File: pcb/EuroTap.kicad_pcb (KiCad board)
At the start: 2 copper layers, 34 x 17 mm, 5 parts, among them J1 AudioJack3_Ground, J2 AudioJack3_Ground, J3 Conn_Coaxial

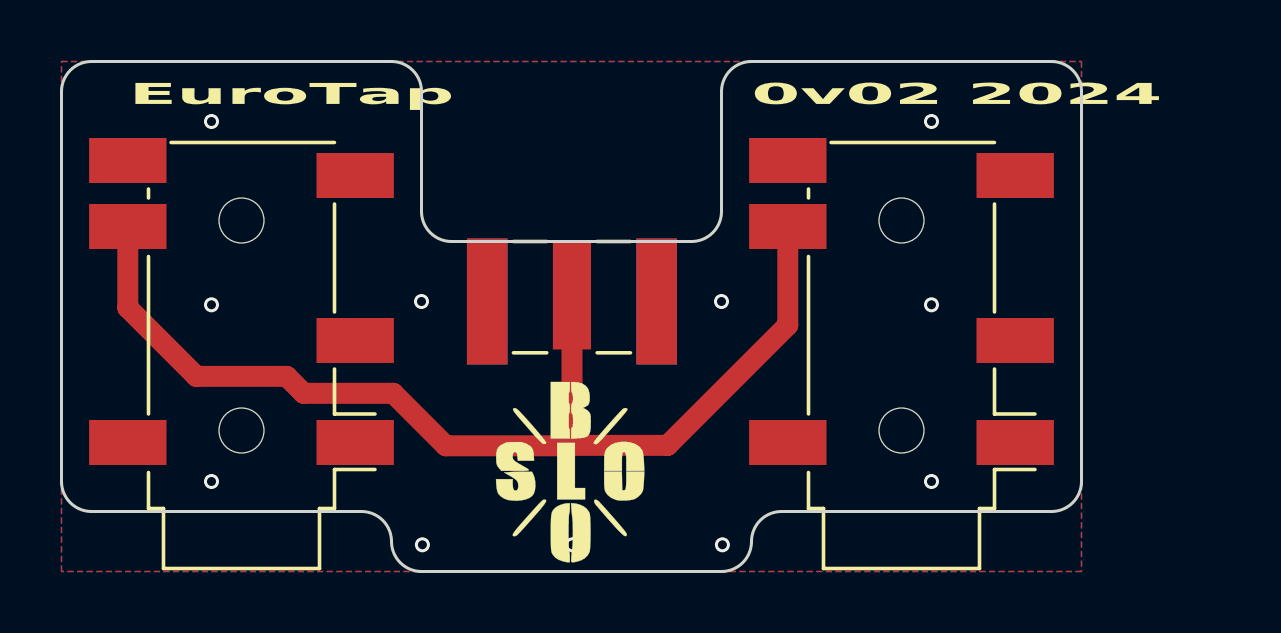
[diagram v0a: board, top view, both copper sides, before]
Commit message: 30cm width
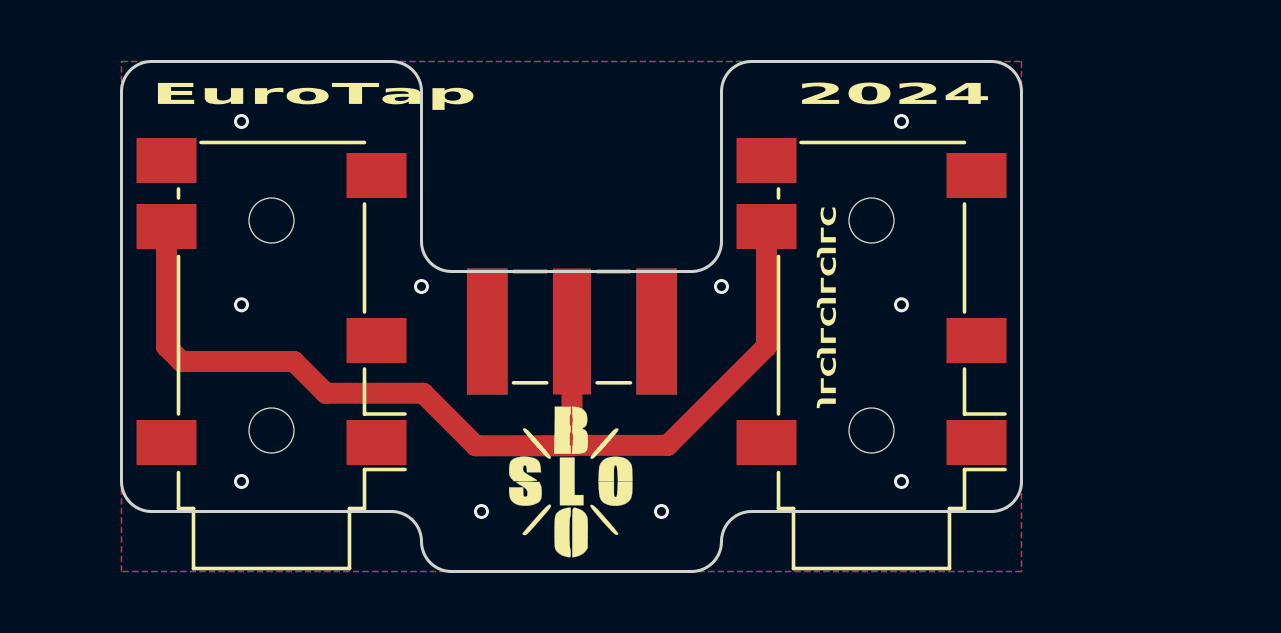
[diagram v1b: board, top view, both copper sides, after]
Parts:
- removed the Ref** at (137.4, 116.7)
- added Ref**: Val**, SloBloLogo, F.Cu at (137.8, 117.5)
- J1, J2: footprint SloBlo:Jack_3.5mm_PJ311_Horizontal_Handsolder -> SloBlo:Jack_3.5mm_PJ311_Horizontal
- moved J1 1.00 mm to (145.0, 108.0)
- moved J2 1.00 mm to (125.0, 108.0)
- moved J3 1.00 mm to (135.0, 109.0)
- moved G*** 0.42 mm to (135.0, 108.5)
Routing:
- net /Signal: track 36.6 -> 34.5 mm
- net GND: vias 11 -> 10
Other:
- board size 34 x 17 mm -> 30 x 17 mm
- board text added: "2024"
- board text removed: "0v02 2024"
